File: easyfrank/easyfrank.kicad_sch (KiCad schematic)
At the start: 4 parts

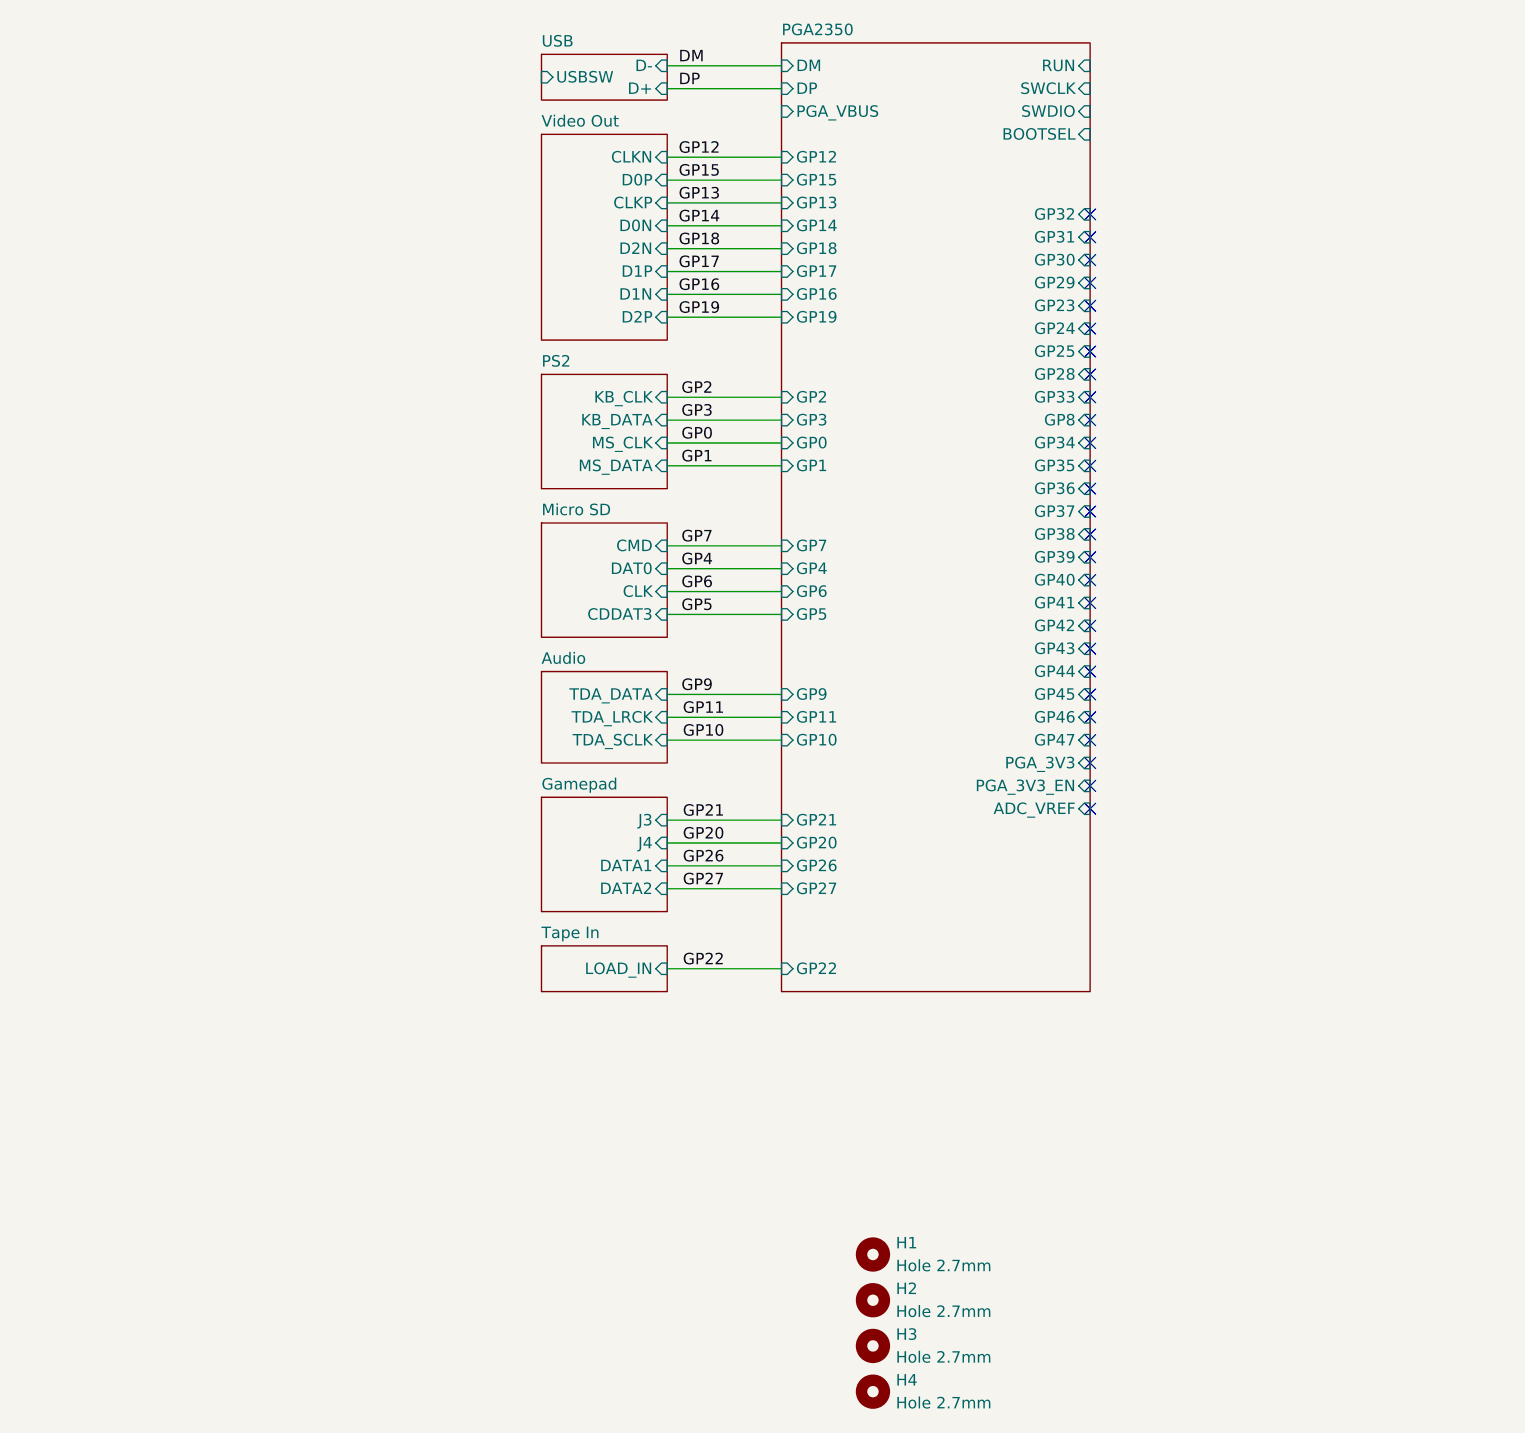
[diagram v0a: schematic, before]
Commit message: EasyFRANK WIP
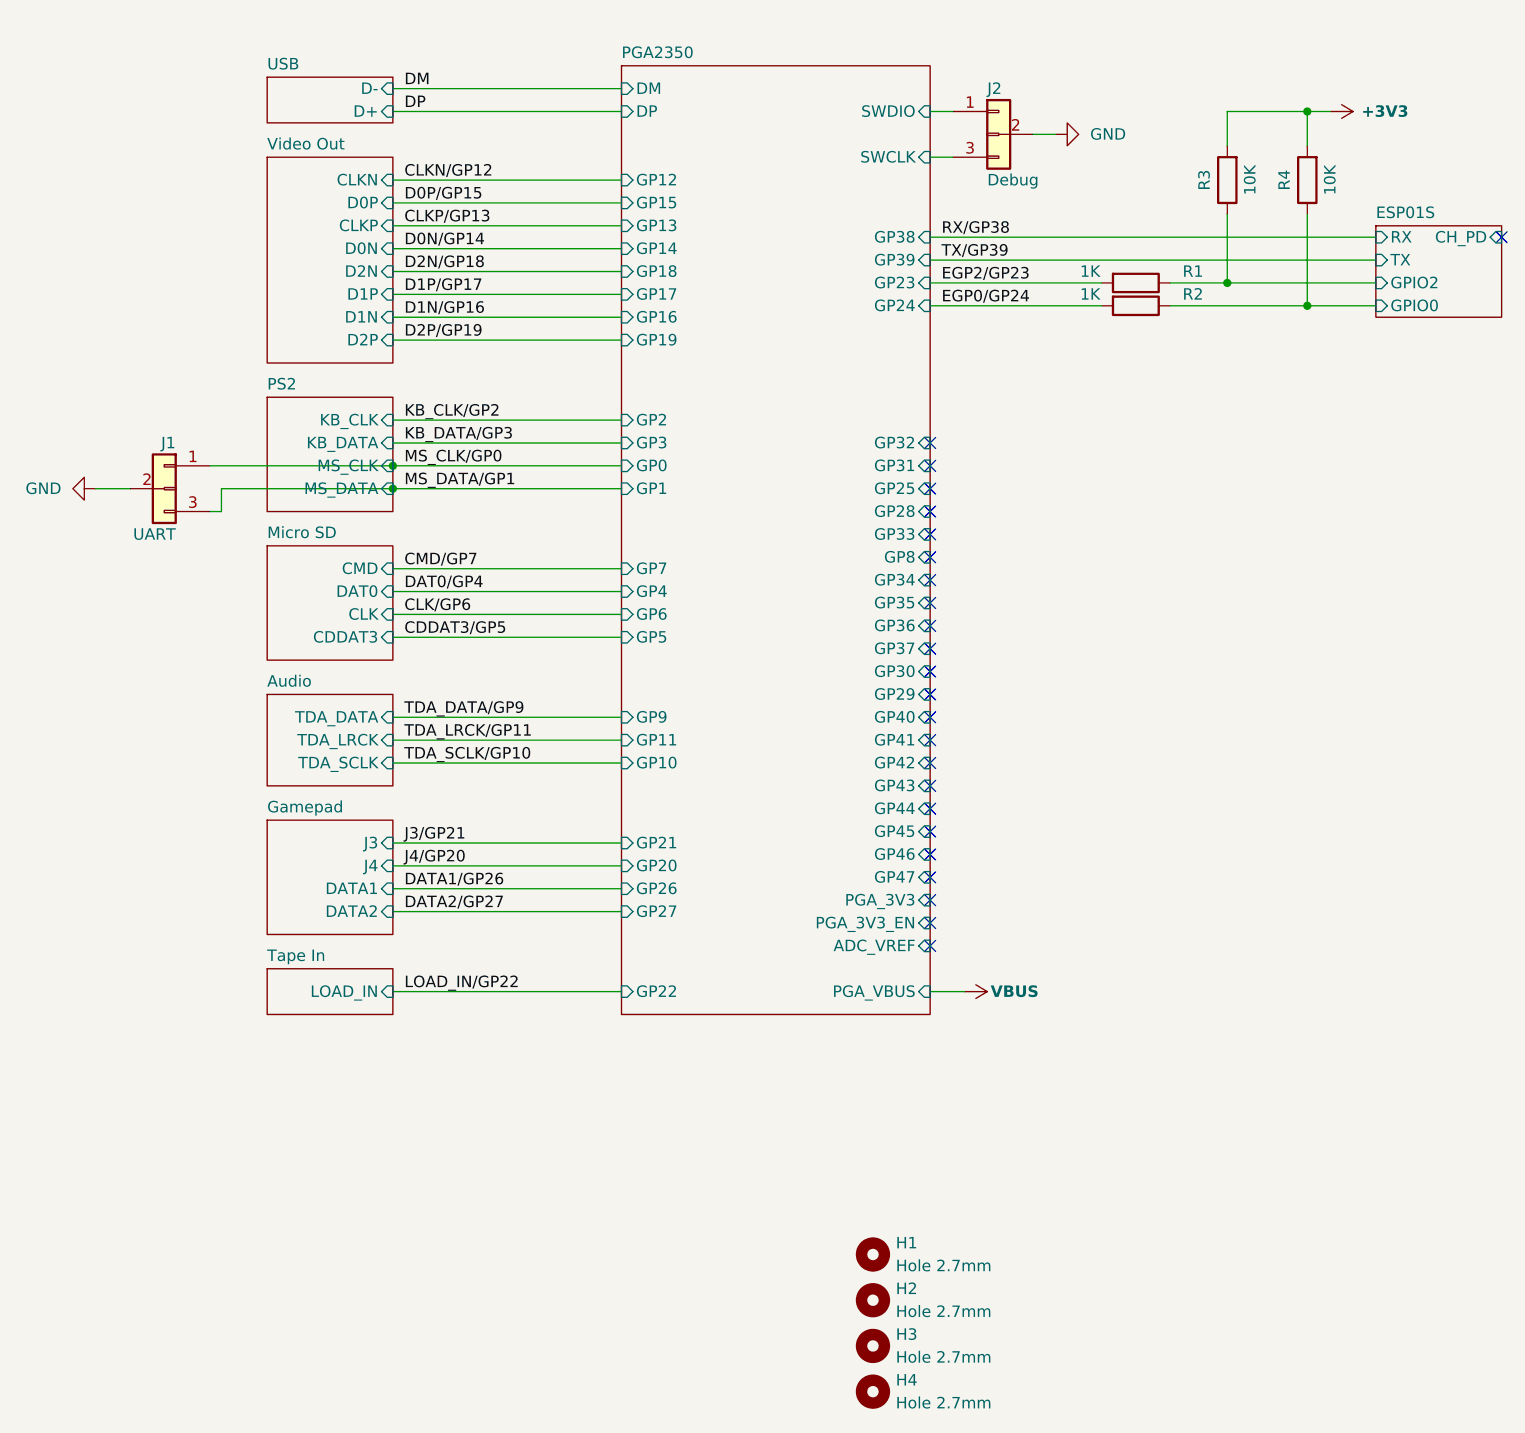
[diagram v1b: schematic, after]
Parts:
- added J1: UART, FRANK:PinSocket_1x03_P2.54mm_Vertical, symbol FRANK:Conn_01x03
- added J2: Debug, FRANK:PinSocket_1x03_P2.54mm_Vertical, symbol FRANK:Conn_01x03
- added R1, R2: 1K, FRANK:Combined_0805_RE, symbol FRANK:R
- added R3, R4: 10K, FRANK:Combined_0805_RE, symbol FRANK:R
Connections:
- net PGA2350/SWCLK: now also J2.3 (Pin_3)
- net PGA2350/SWDIO: now also J2.1 (Pin_1)
- new net +3V3: R3.2, R4.2
- new net EGP0/GP24: R2.2
- new net EGP2/GP23: R1.2
- new net ESP01S/GPIO0: R2.1, R4.1
- new net ESP01S/GPIO2: R1.1, R3.1
- new net GND: J1.2 (Pin_2), J2.2 (Pin_2)
- new net MS_CLK/GP0: J1.1 (Pin_1)
- new net MS_DATA/GP1: J1.3 (Pin_3)
- no-connect marks 27 -> 24
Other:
- added sheet ESP01S (esp01s.kicad_sch)
- sheet PGA2350 ports: added none; removed BOOTSEL, RUN
- sheet USB ports: added none; removed USBSW
